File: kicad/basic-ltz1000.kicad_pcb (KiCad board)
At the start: 2 copper layers, 49.5 x 49.5 mm, 44 parts, among them P1 CONN_1X1, P2 CONN_1X1, P3 CONN_1X1, P4 CONN_1X1, P5 CONN_1X1, P6 CONN_2X1, Q1 2N3904, U1 LTZ1000A, U2 LT1013, U30 LTC2057

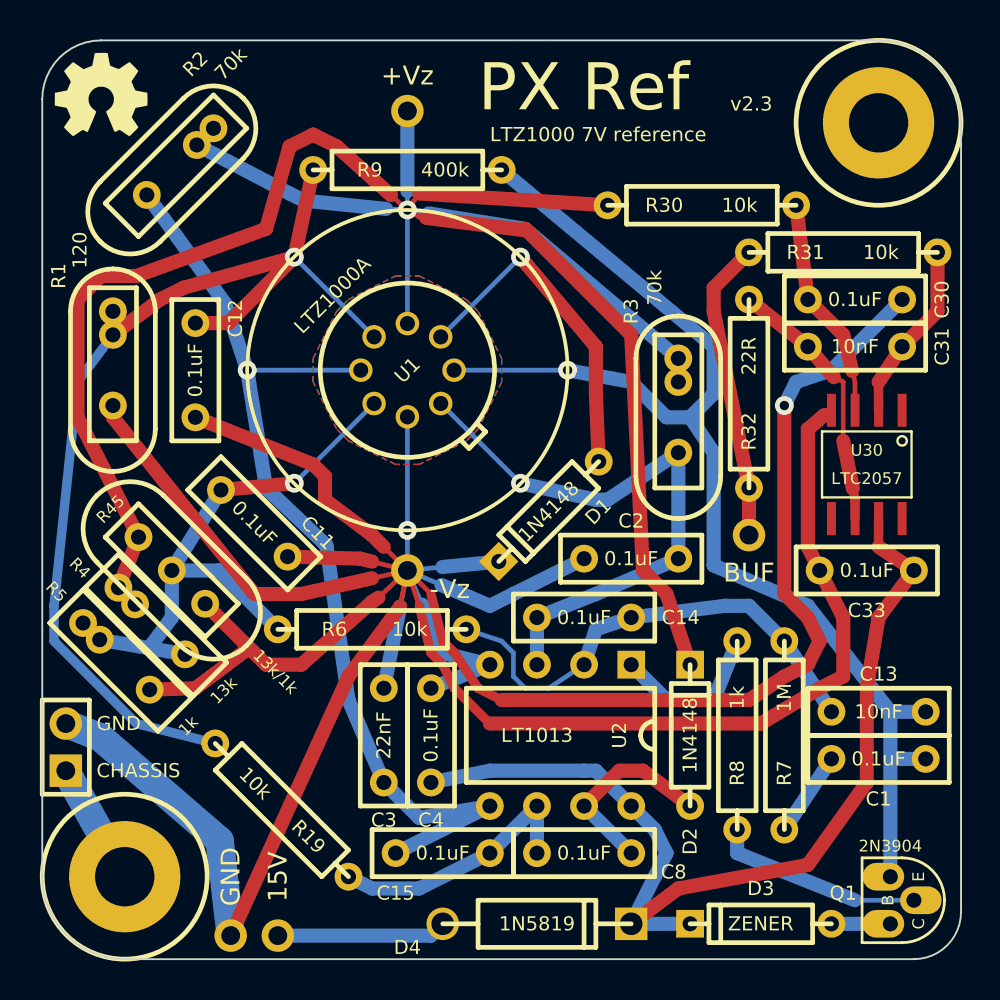
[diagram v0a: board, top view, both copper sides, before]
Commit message: v2.4 gerbers
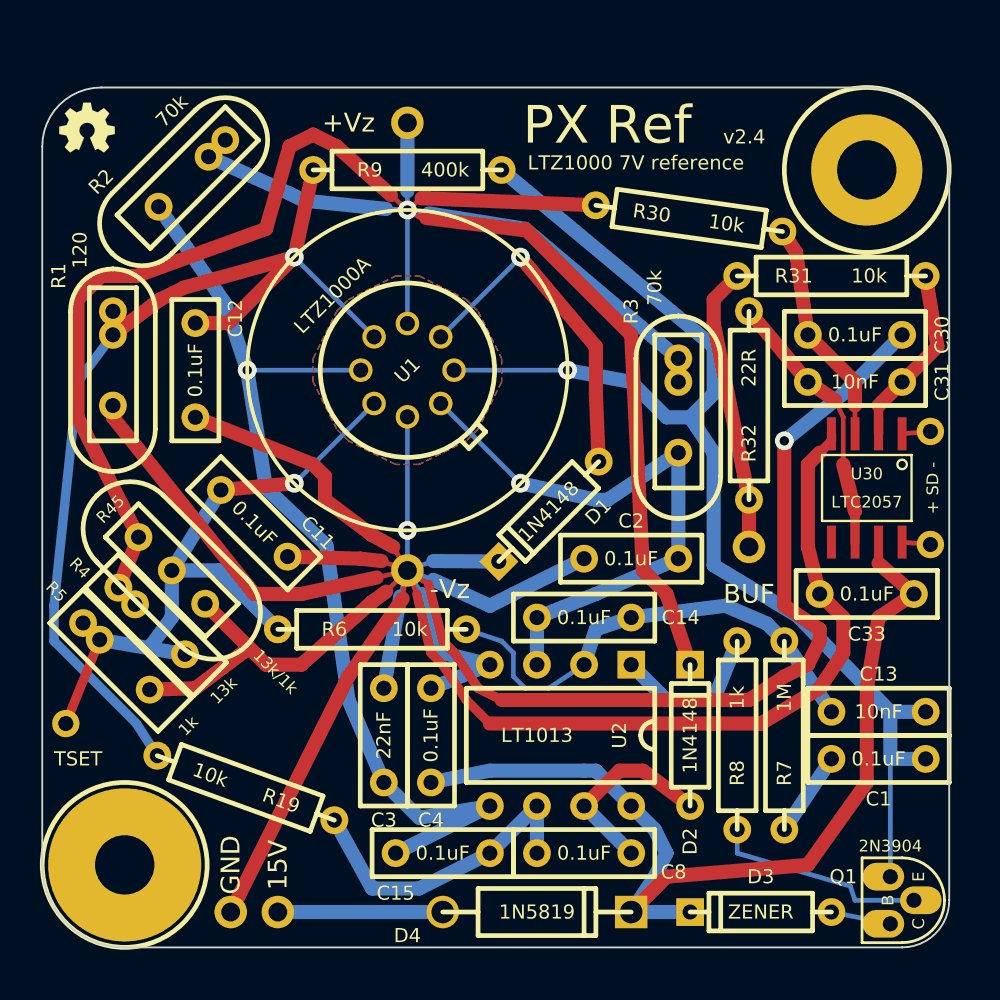
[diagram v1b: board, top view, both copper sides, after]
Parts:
- removed the G*** at (201.3, 67.7)
- removed P6: CONN_2X1, SIL-2
- added G***: OSHW-logo_silkscreen-front_3mm, OSHW-logo_silkscreen-front_3mm, F.Cu at (200.5, 69.5)
- added H***: Val**, 1pin_032_058, F.Cu at (246.0, 85.9)
- added H***: Val**, 1pin_032_058, F.Cu at (246.0, 91.9)
- added H***: Val**, 1pin_032_058, F.Cu at (199.4, 101.6)
- moved R19 3.14 mm to (213.9, 106.8), turned to 160 degrees
- moved H*** 2.62 mm to (242.6, 71.8)
- moved C30 1.91 mm to (241.9, 80.6)
- moved C31 1.91 mm to (241.9, 83.2)
- moved R31 1.42 mm to (245.7, 77.5)
- moved U30 1.27 mm to (242.6, 88.9)
- moved C33 1.27 mm to (242.6, 94.6)
- moved P1 1.27 mm to (210.8, 111.8)
- moved P4 1.27 mm to (208.3, 111.8)
- moved R2 0.90 mm to (205.7, 72.4)
- moved H1 0.64 mm to (202.6, 109.2)
- moved P2 0.64 mm to (217.8, 69.2)
- moved P3 0.64 mm to (236.2, 92.1)
- moved R32 0.64 mm to (236.2, 79.4)
- moved D3 0.63 mm to (236.9, 111.8)
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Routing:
- net Vz- Sense: track 240.1 -> 220.2 mm
- net (no net): track 0.00 -> 7.94 mm
- net CHASSIS: track 6.54 -> 0.00 mm
- net N-000007: track 14.4 -> 17.1 mm
- net 15V: track 54.0 -> 51.6 mm
- net Vz+ Sense: track 129.3 -> 127.0 mm
- net N-0000023: track 57.8 -> 55.5 mm
- net N-0000012: track 14.2 -> 15.8 mm
- net Vz+ Buf: track 16.2 -> 15.3 mm
- net N-0000014: track 53.5 -> 52.7 mm
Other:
- board size 49.5 x 49.5 mm -> 48.9 x 46.4 mm
- board text added: "+ SD -"
- board text added: "TSET"
- board text added: "v2.4"
- board text removed: "CHASSIS"
- board text removed: "v2.3"
